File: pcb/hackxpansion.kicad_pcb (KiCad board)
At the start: 4 copper layers, 52 x 43 mm, 69 parts, among them CN2 533981471, CN3 533981471, IC1 ADS7128IRTET, J1 Conn_01x03_MountingPin, J2 USB_C_Receptacle_USB2.0_14P, Q1 BSS138, Q2 2N7002, SW1 SW_Push, SW2 SW_Push, SW3 SW_On_Off, U2 RP2354B, U5 SPX3819M5-L-3-3, U7 BQ24075RGT, Y1 ABM8-272-T3

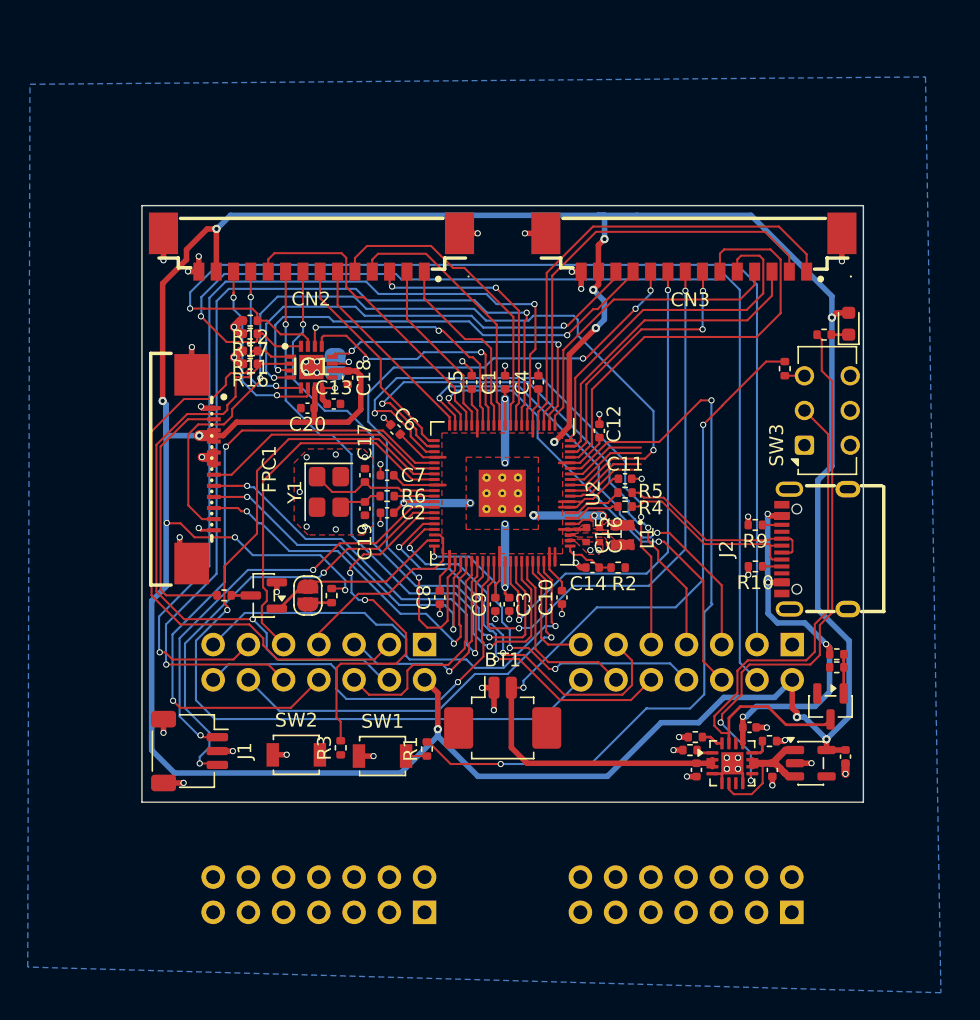
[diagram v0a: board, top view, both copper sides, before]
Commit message: cleaned up routing
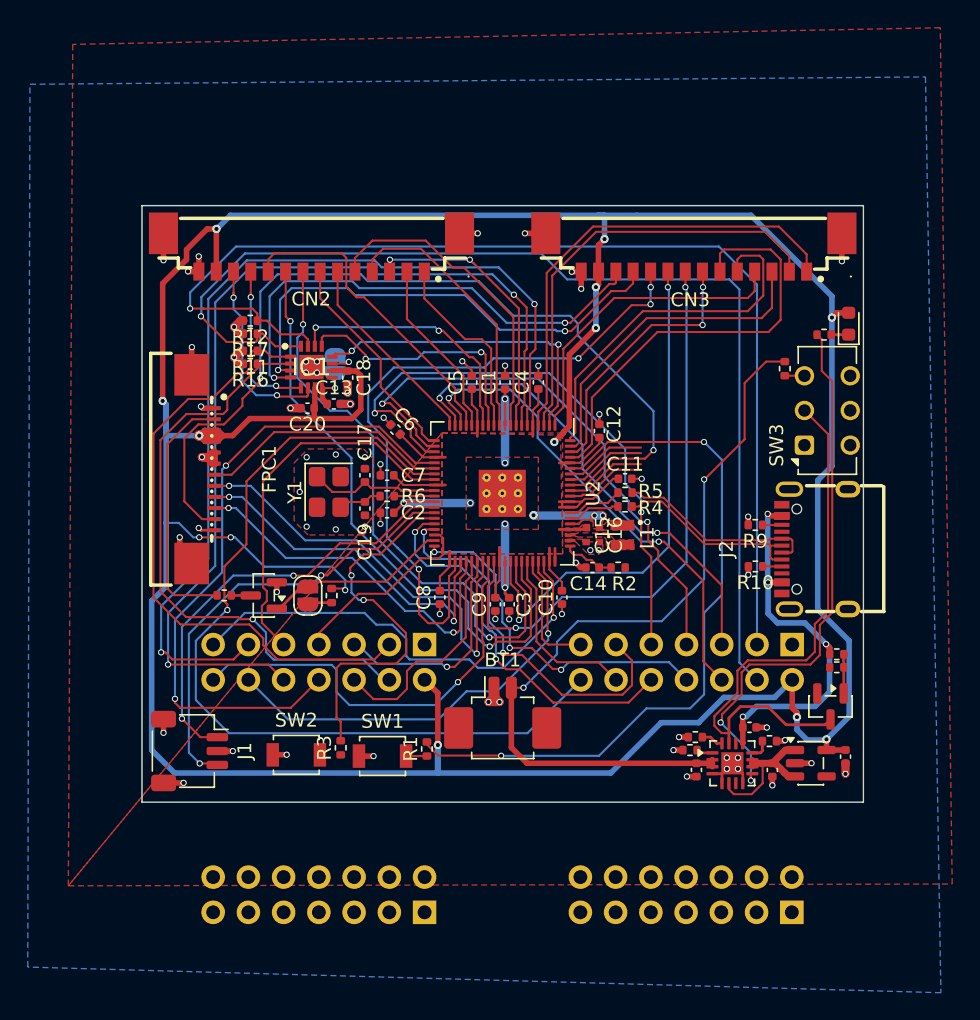
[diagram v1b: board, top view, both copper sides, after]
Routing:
- net /+3V3: track 289.9 -> 295.4 mm
- net /Main Board/RP2354B/QSPI_SS: track 56.5 -> 52.0 mm
- net /Connector Main Mod2/mod.MD0: track 32.8 -> 35.4 mm
- net /Connector Main Mod2/mod.MD1: track 33.6 -> 35.9 mm
- net /GND: track 54.4 -> 56.5 mm, vias 63 -> 66
- net /Main Board/Display/RESET: track 62.4 -> 64.4 mm
- net /Connector Main Mod2/bank.GPIO8: track 38.9 -> 37.4 mm
- net /Main Board/Module Bay 0/GPIO5: track 68.3 -> 69.6 mm
- net /Main Board/Display/SCLK: track 27.0 -> 25.9 mm
- net /Main Board/Display/MOSI: track 27.8 -> 26.7 mm
- net /Main Board/Module Bay 0/GPIO6: track 67.7 -> 68.9 mm
- net /Main Board/ADC/mod1.MD0: track 79.6 -> 80.7 mm
- net /Main Board/Module Bay 1/GPIO9: track 62.8 -> 63.7 mm
- net Net-(FPC1-Pad2): track 19.2 -> 18.3 mm
- net /Connector Main Mod3/bank.GPIO8: track 44.7 -> 43.8 mm
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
